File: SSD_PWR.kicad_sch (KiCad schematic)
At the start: 48 parts, among them U10 TPS54335-1ADRCT, U8 TPS54335-1ADRCT, U9 TPS54335-1ADRCT

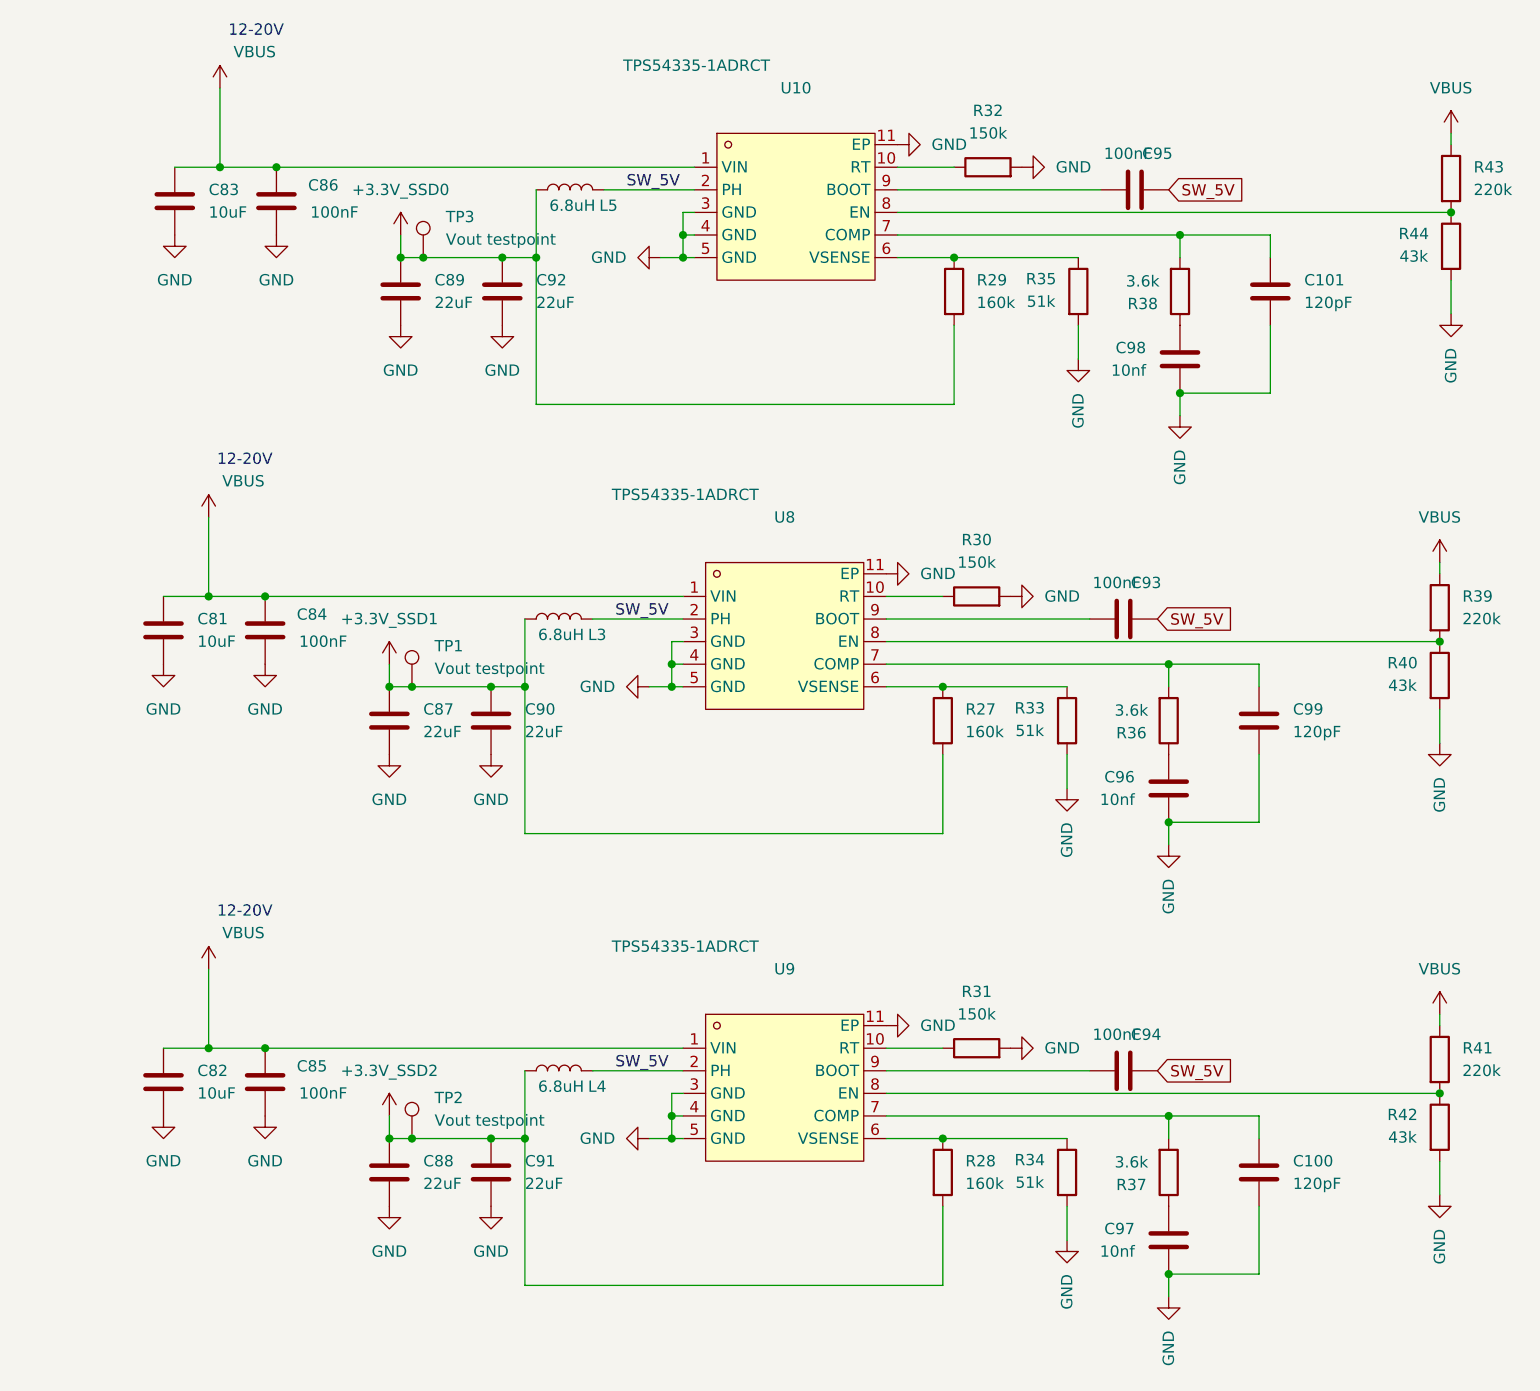
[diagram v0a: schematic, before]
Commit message: .
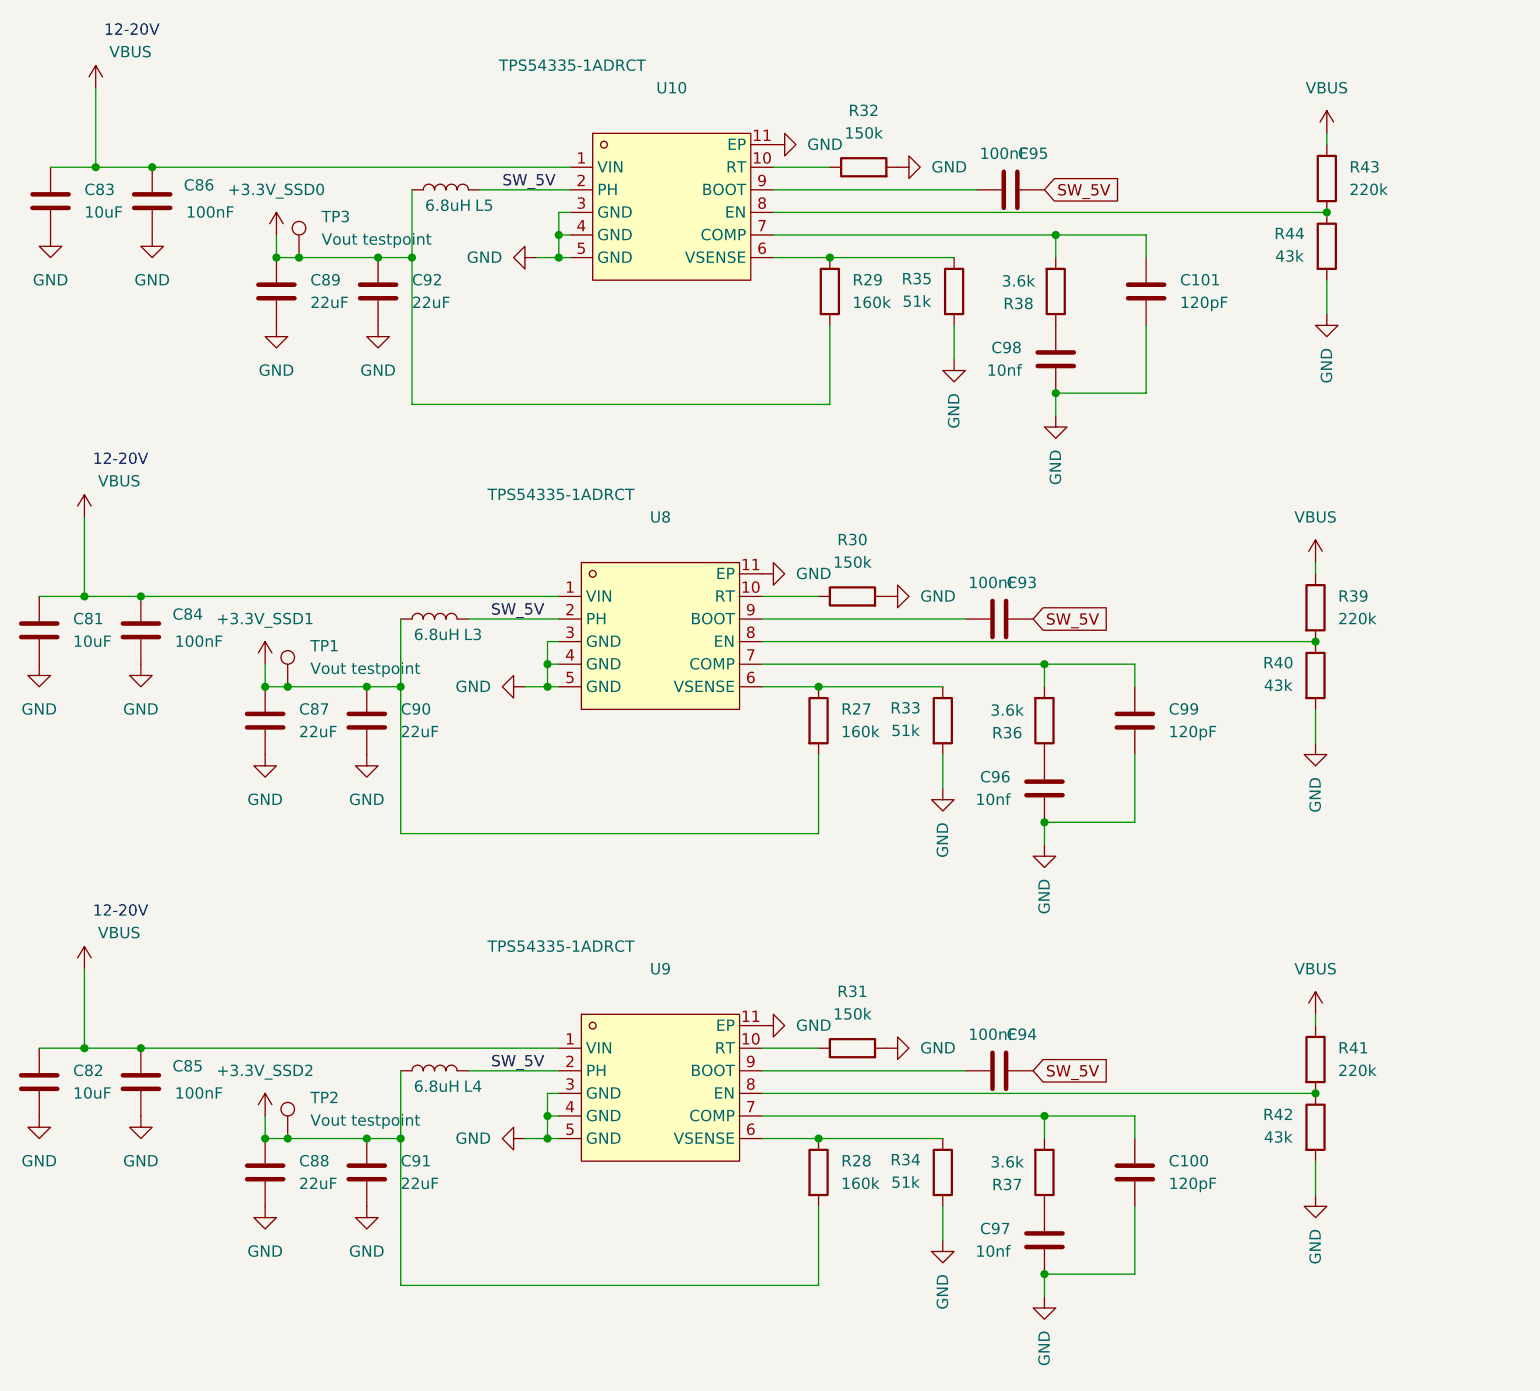
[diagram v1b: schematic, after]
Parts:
- L3, L4, L5: footprint easyeda2kicad:IND-SMD_L12.0-W12.0 -> Inductor_SMD:L_APV_APH0530
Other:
- moved on the sheet: C100, C101, C81, C82, C83, C84, C85, C86, C87, C88, C89, C90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
